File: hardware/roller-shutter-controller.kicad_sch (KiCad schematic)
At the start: 37 parts, among them J1 Screw_Terminal_01x06, J2 Screw_Terminal_01x04, J3 Screw_Terminal_01x10, K1 EC2-3NU, Q1 2N7002, Q2 2N7002, Q3 2N7002, U1 TSR_1-24120, U2 TSR_1-2433, U3 WeMos_C3_mini, U4 ESP32-C3-WROOM-02U

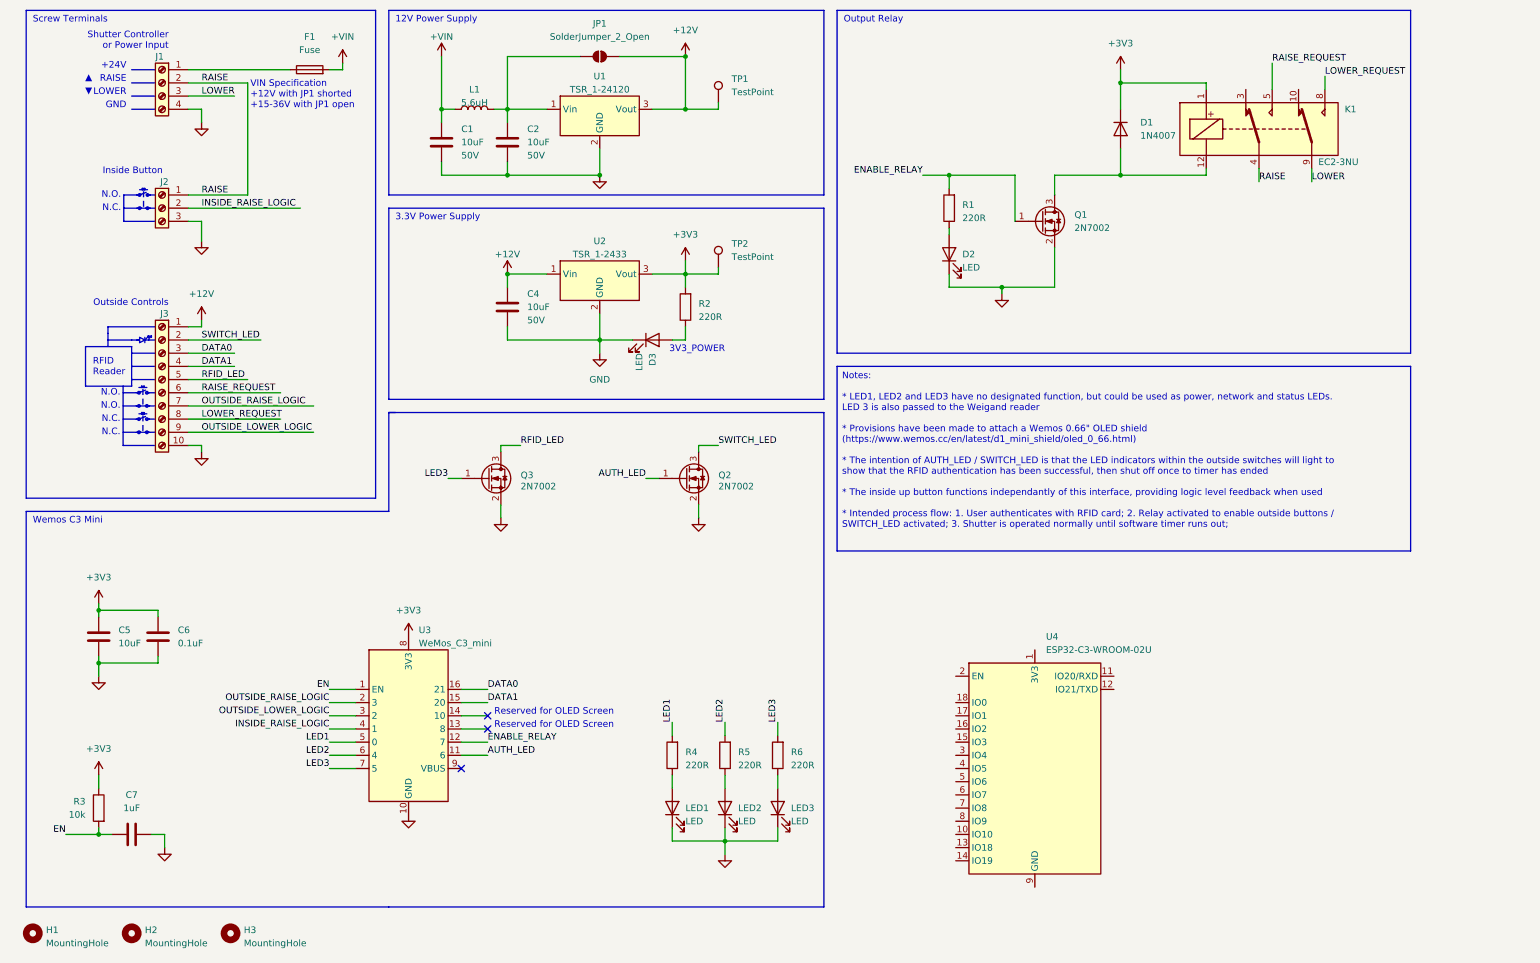
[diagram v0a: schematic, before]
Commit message: first draft of v4 schematic
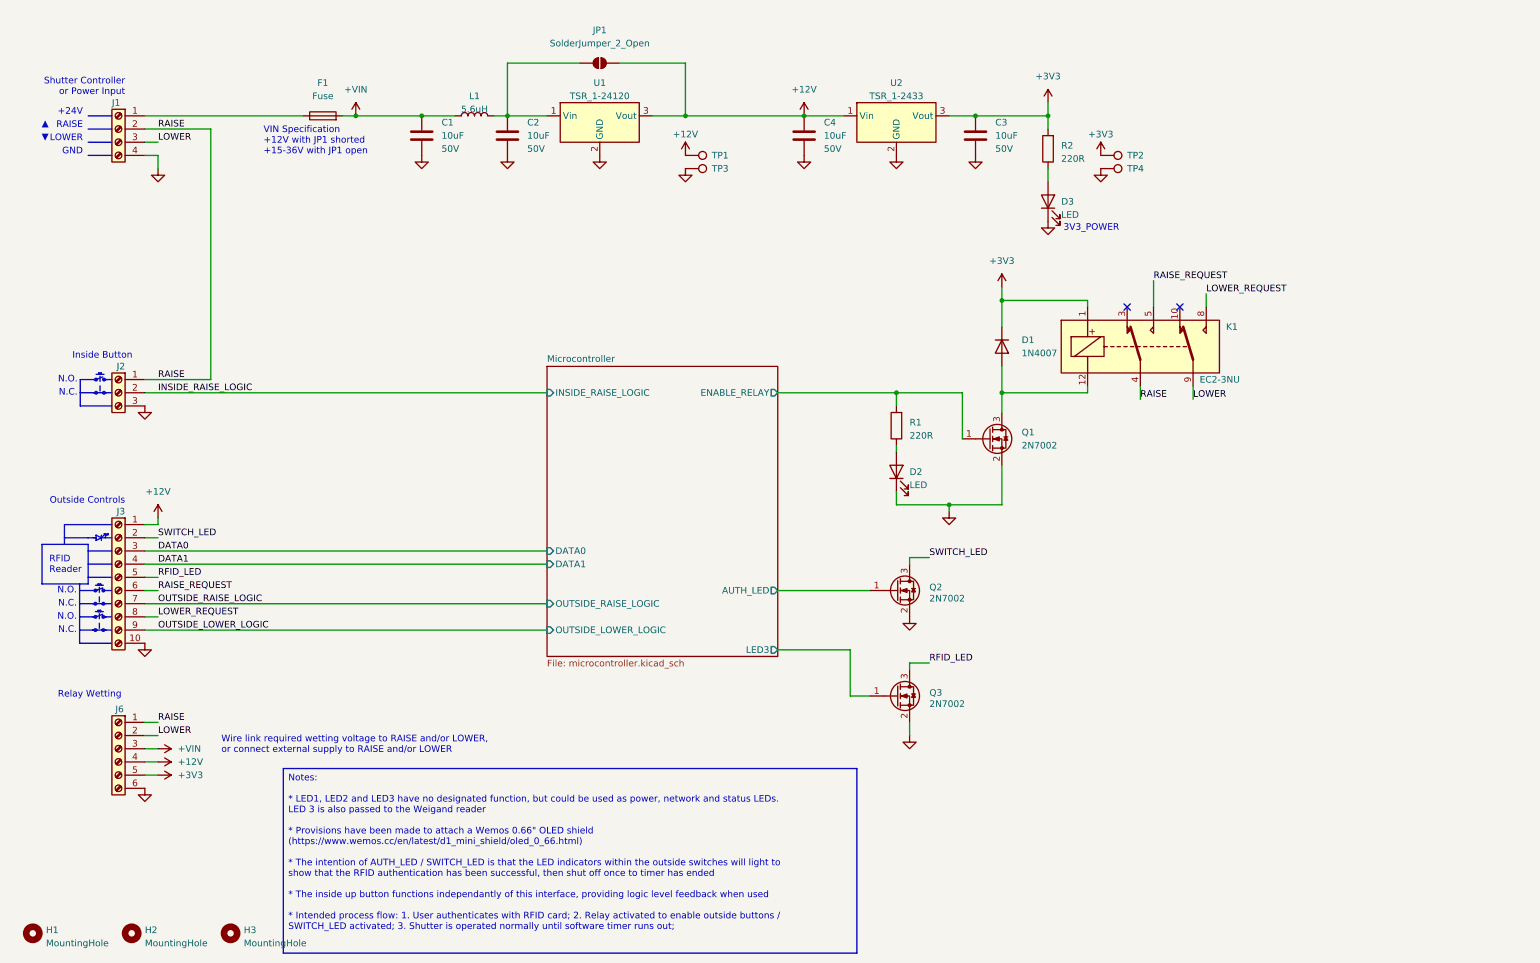
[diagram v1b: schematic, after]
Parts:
- removed C5: 10uF, Capacitor_SMD:C_1210_3225Metric_Pad1.33x2.70mm_HandSolder, symbol Device:C
- removed C6: 0.1uF, Capacitor_SMD:C_0603_1608Metric_Pad1.08x0.95mm_HandSolder, symbol Device:C
- removed C7: 1uF, Capacitor_SMD:C_0603_1608Metric_Pad1.08x0.95mm_HandSolder, symbol Device:C
- removed LED1, LED2, LED3: LED, LED_SMD:LED_0603_1608Metric_Pad1.05x0.95mm_HandSolder, symbol Device:LED
- removed R3: 10k, Resistor_SMD:R_0603_1608Metric_Pad0.98x0.95mm_HandSolder, symbol Device:R
- removed R4, R5, R6: 220R, Resistor_SMD:R_0603_1608Metric_Pad0.98x0.95mm_HandSolder, symbol Device:R
- removed U3: WeMos_C3_mini, Lolin C3 Mini:wemos-d1-mini-with-pin-header-and-connector, symbol Custom:WeMos_C3_mini
- removed U4: ESP32-C3-WROOM-02U, RF_Module:ESP32-C3-WROOM-02U, symbol RF_Module:ESP32-C3-WROOM-02U
- added C3: 10uF, Capacitor_SMD:C_1210_3225Metric_Pad1.33x2.70mm_HandSolder, symbol Device:C
- added J6: Screw_Terminal_01x06, symbol Connector:Screw_Terminal_01x06
- added TP3, TP4: TestPoint, TestPoint:TestPoint_Pad_1.0x1.0mm, symbol Connector:TestPoint
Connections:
- net +12V: now also J6.4 (Pin_4)
- net +3V3: now also C3.1, J6.5 (Pin_5)
- net +VIN: now also J6.3 (Pin_3)
- net GND: now also C3.2, J6.6 (Pin_6), TP3.1, TP4.1
- net LOWER: now also J6.2 (Pin_2)
- net RAISE: now also J6.1 (Pin_1)
- net AUTH_LED renamed Microcontroller/AUTH_LED
- net ENABLE_RELAY renamed Microcontroller/ENABLE_RELAY
- net LED3 renamed Microcontroller/LED3
- no-connect marks 3 -> 2
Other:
- added sheet Microcontroller (microcontroller.kicad_sch)
- note added: "Relay Wetting"
- note added: "Wire link required wetting voltage to RAISE and/or LOWER, or connect external supply to RAISE and/or LOWER"
- note removed: "12V Power Supply"
- note removed: "3.3V Power Supply"
- note removed: "Output Relay"
- note removed: "Reserved for OLED Screen"
- note removed: "Screw Terminals"
- note removed: "Wemos C3 Mini"
- moved on the sheet: C1, C2, C4, D1, D2, D3, F1, J1, J2, J3, JP1, K1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
